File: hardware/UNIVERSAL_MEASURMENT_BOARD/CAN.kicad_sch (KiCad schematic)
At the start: 18 parts, among them U14 ADM3055EBRIZ-RL

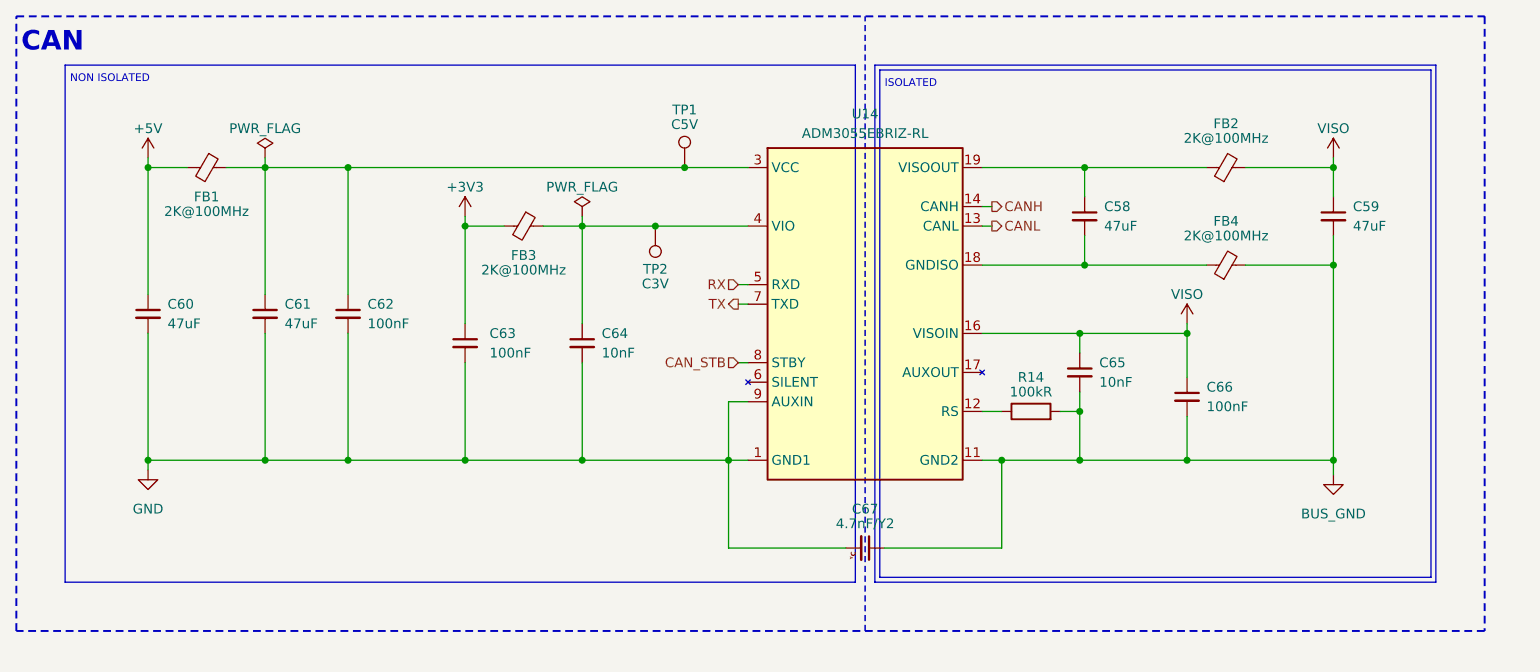
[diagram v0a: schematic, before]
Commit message: final schematic review corrections
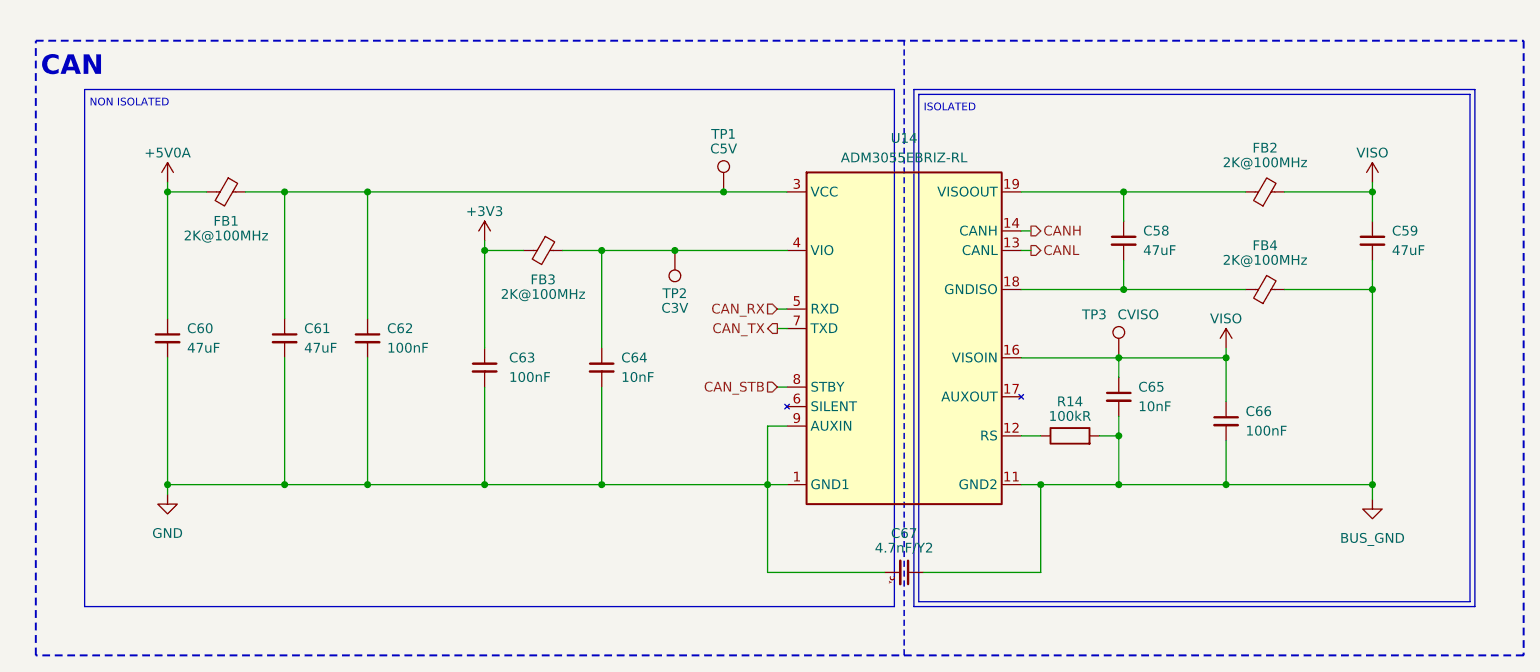
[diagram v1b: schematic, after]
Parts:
- added TP3: CVISO, symbol Connector:TestPoint
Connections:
- net VISO: now also TP3.1
- net +5V renamed +5V0A
- net RX renamed CAN_RX
- net TX renamed CAN_TX
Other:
- moved on the sheet: C58, C59, C60, C61, C62, C63, C64, C65, C66, C67, FB1, FB2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
